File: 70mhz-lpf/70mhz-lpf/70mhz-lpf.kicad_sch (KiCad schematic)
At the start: 16 parts, among them J701 Coax Solder Point, J702 Coax Solder Point

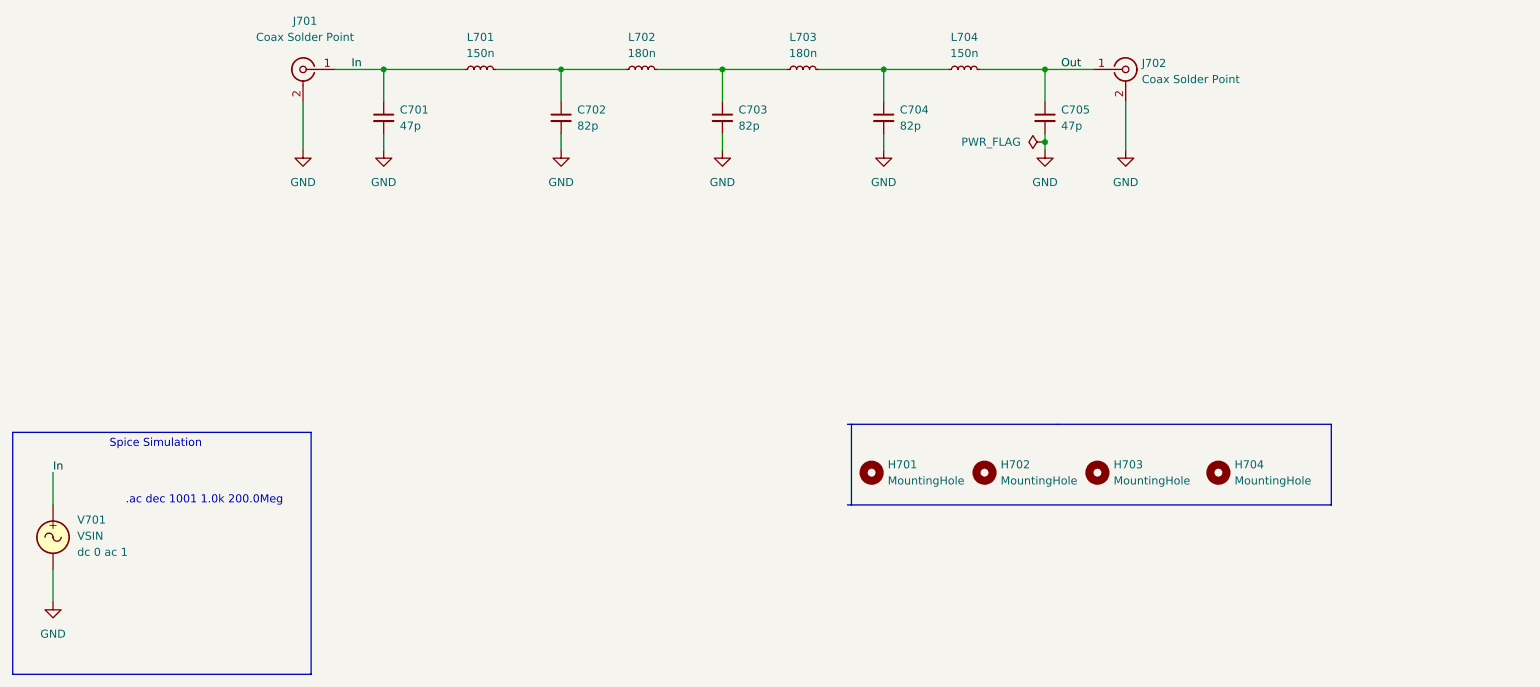
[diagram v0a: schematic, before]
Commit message: v7 conversion
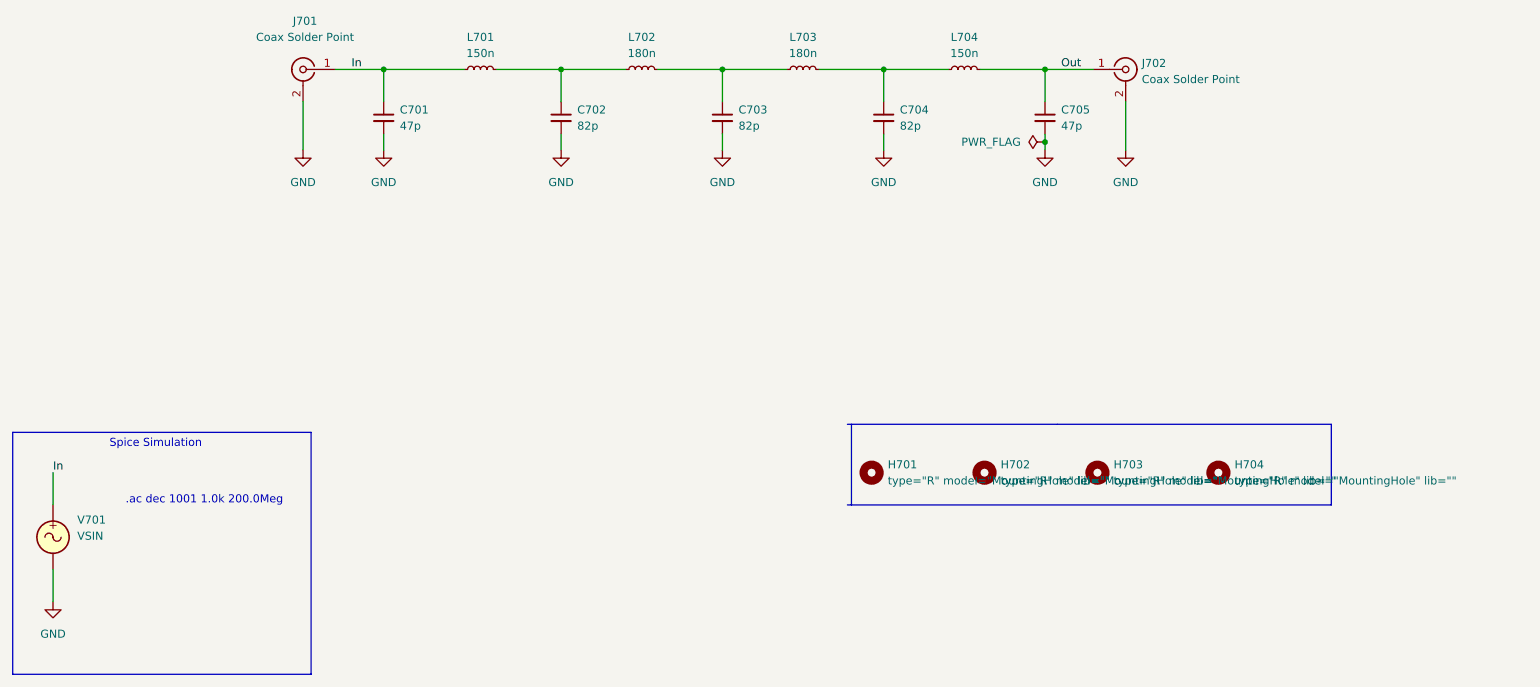
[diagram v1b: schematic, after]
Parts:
- H701, H702, H703, H704: value MountingHole -> ${SIM.PARAMS}; Spice_Netlist_Enabled N -> (none); Spice_Primitive R -> (none)
- J701, J702: Spice_Model Conn_Coaxial -> (none); Spice_Netlist_Enabled N -> (none); Spice_Primitive J -> (none)
- V701: Spice_Model dc 0 ac 1 -> (none); Spice_Netlist_Enabled Y -> (none); Spice_Primitive V -> (none)
